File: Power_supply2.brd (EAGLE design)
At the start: 84.4 x 61.4 mm, 34 parts, among them IC1 7808T, IC2 7812T, IC3 7808T, IC4 7808T, IC5 7808T, IC6 7808T

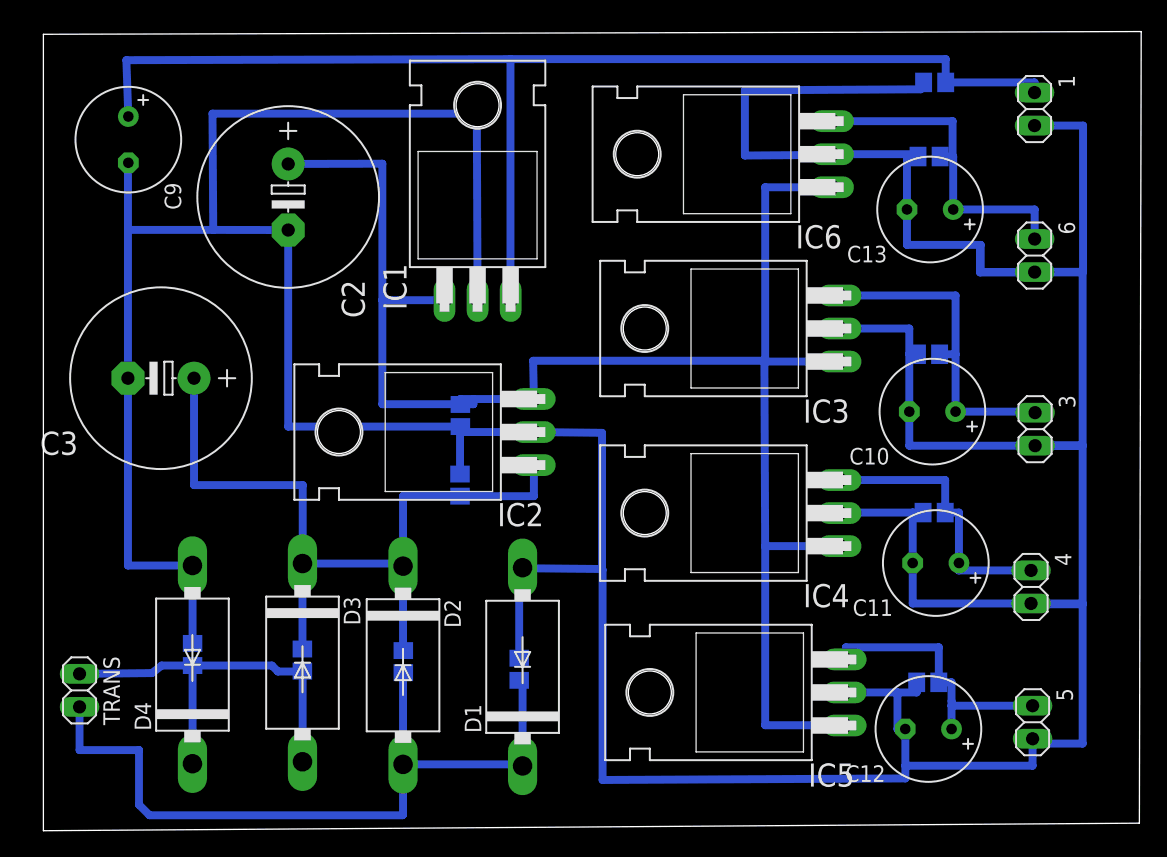
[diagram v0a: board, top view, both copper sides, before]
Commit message: Modofied SCH & BRD
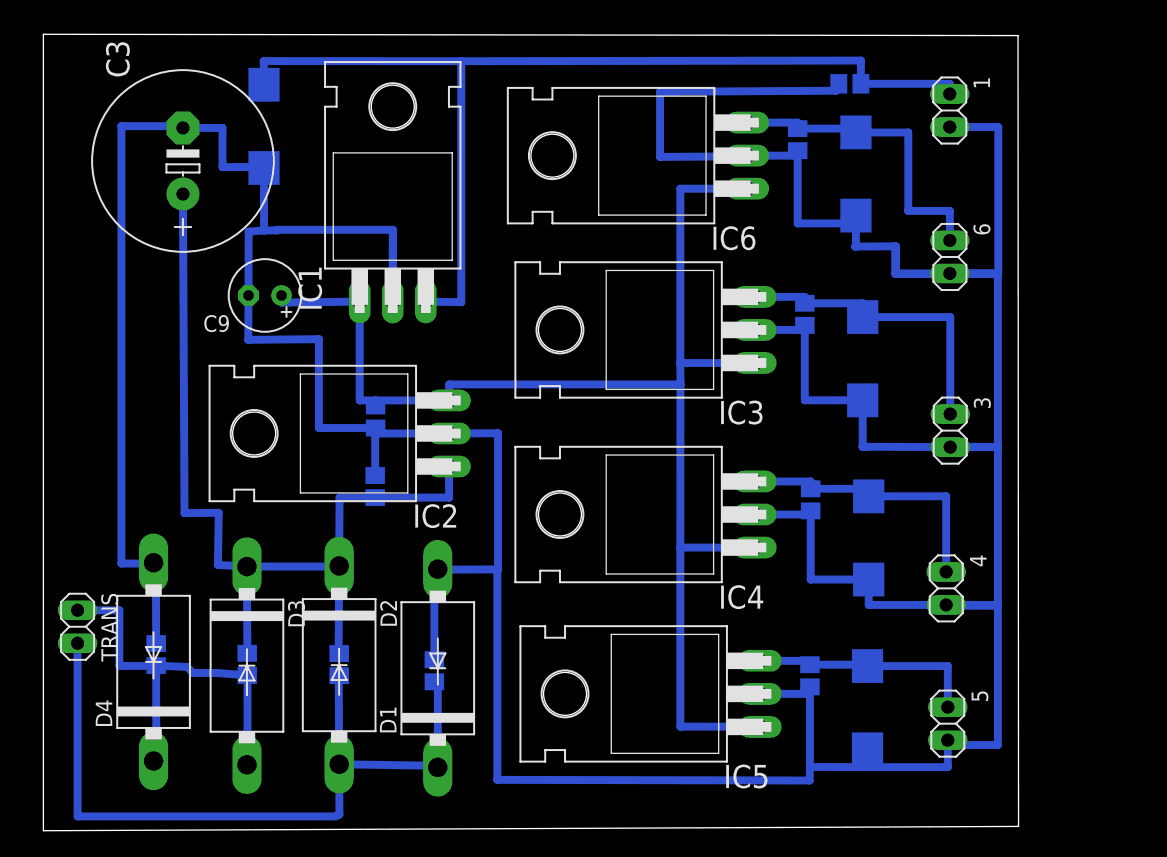
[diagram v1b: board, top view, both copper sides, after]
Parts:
- removed C10, C11, C12, C13: 10u, resistor:E3,5-8
- removed C2: 100u, resistor:E5-13
- added C19, C20, C21, C22, C23: 10u, resistor:CT7343
- C3: value 100u -> 1000u
- C9: value 10u -> 100u; device resistor:E3,5-8 -> resistor:E2,5-6
- moved C3 16.8 mm to (10.7, 51.5), turned to 90 degrees
- moved C9 15.9 mm to (17.0, 41.1), turned to 180 degrees
- moved C8 10.2 mm to (58.0, 53.1), turned to 270 degrees
- moved C5 9.99 mm to (58.5, 39.7), turned to 270 degrees
- moved C6 9.54 mm to (59.0, 25.4), turned to 270 degrees
- moved C7 9.07 mm to (58.9, 11.9), turned to 270 degrees
- moved 4 6.52 mm to (69.4, 18.6)
- moved C1 6.52 mm to (25.5, 31.8)
- moved D1 6.52 mm to (30.3, 12.5)
- moved IC1 6.52 mm to (26.9, 50.8)
- moved IC3 6.52 mm to (44.5, 38.5)
- moved IC4 6.52 mm to (44.5, 24.3)
- moved IC5 6.52 mm to (44.9, 10.5)
- moved C14 6.52 mm to (25.5, 26.5)
- moved C16 6.52 mm to (30.1, 12.3)
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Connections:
- net GND: now also C19.-, C20.-, C21.-, C22.-, C23.-; no longer C10.-, C11.-, C12.-, C13.-, C2.-
- net N$2: now also C21.+; no longer C11.+
- net N$3: now also C22.+; no longer C12.+
- net N$4: now also C19.+; no longer C9.+
- net N$5: now also C9.+; no longer C2.+
- net N$6: now also C20.+; no longer C10.+
- net N$7: now also C23.+; no longer C13.+
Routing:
- net N$5: track 129.0 -> 104.6 mm
- net GND: track 413.6 -> 393.1 mm
- net N$4: track 95.3 -> 78.4 mm
- net N$10: track 61.5 -> 70.3 mm
- net N$3: track 21.6 -> 18.0 mm
- net N$6: track 25.3 -> 24.0 mm
- net N$9: track 59.8 -> 58.7 mm
- net N$7: track 25.6 -> 24.6 mm
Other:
- board size 84.4 x 61.4 mm -> 75 x 61.2 mm
